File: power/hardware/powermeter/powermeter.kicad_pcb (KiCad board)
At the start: 2 copper layers, 34.6 x 35.6 mm, 20 parts, among them J1 Conn_01x02_Socket, J2 Conn_01x04_Pin, J3 Conn_01x02_Socket, P1 USB_C_Plug_USB2.0, U2 ESP32-S3-WROOM-1, U3 AZ1117-3.3

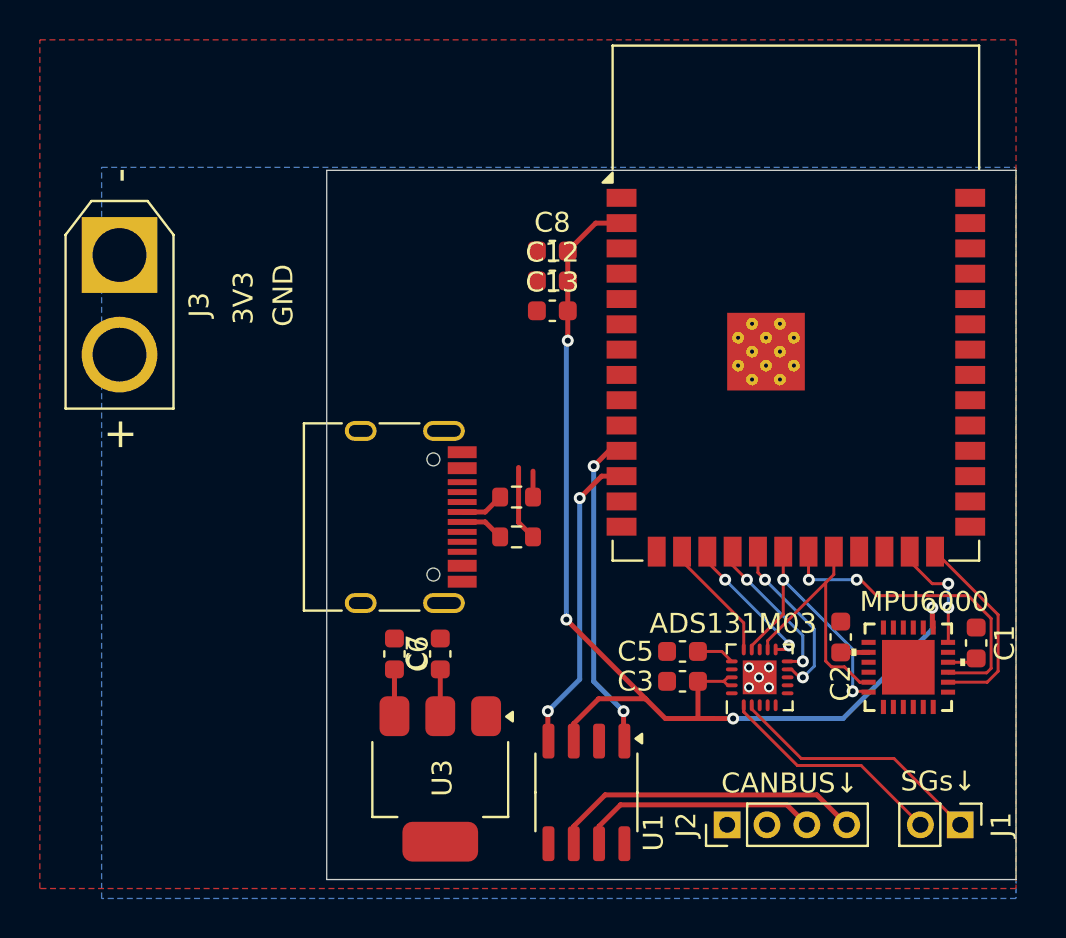
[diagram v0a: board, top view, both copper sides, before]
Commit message: updated pcb
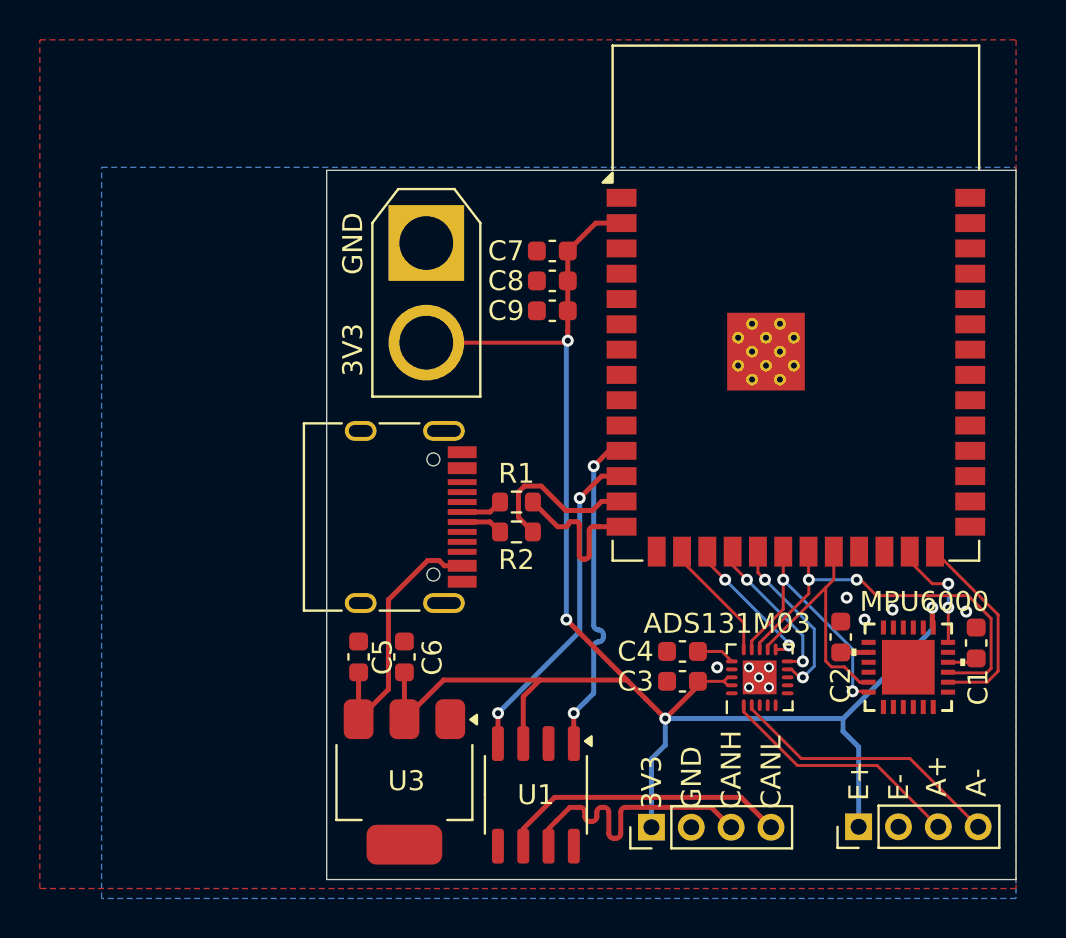
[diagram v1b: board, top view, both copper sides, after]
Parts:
- removed J1: Conn_01x02_Socket, Connector_PinHeader_2.00mm:PinHeader_1x02_P2.00mm_Vertical
- added J4: Conn_01x04_Pin, Connector_PinHeader_2.00mm:PinHeader_1x04_P2.00mm_Vertical, F.Cu at (181.5, 89.9)
- moved J3 15.4 mm to (159.8, 60.6)
- moved J2 3.80 mm to (171.1, 89.9)
- moved U1 2.54 mm to (165.3, 88.3)
- moved C6 1.81 mm to (158.7, 81.4)
- moved U3 1.81 mm to (158.7, 87.7)
- moved C5 1.81 mm to (156.4, 81.4)
- moved R1 0.25 mm to (164.3, 73.6)
- moved R2 0.25 mm to (164.3, 75.1)
- renumbered C5 to C4, C6 to C5, C7 to C6, C8 to C7, C12 to C8, C13 to C9
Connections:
- ADS131M03 pad 21: (no net) -> GND
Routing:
- net +3V3: track 58.1 -> 87.1 mm
- net +5V: track 2.49 -> 13.6 mm
- net /USB_{D}+: track 1.30 -> 8.26 mm
- net /MISO: track 16.1 -> 20.7 mm
- net /USB_{D}-: track 3.79 -> 8.30 mm
- net /CANL: track 15.8 -> 13.7 mm
- net /RX: track 14.8 -> 16.6 mm
- net /CANH: track 12.2 -> 13.6 mm
- net /TX: track 15.6 -> 16.6 mm
- net /ADS+: track 11.5 -> 12.5 mm
- net /ADS-: track 13.1 -> 14.0 mm
- net GND: track 0.00 -> 0.04 mm, vias 5 -> 10
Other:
- board text added: "3 power sources: - 5V USB - 3.3V wired - external battery"
- board text added: "A+"
- board text added: "A-"
- board text added: "CANH"
- board text added: "CANL"
- board text added: "E+"
- board text added: "E-"
- board text added: "is AdS131 vdd And dvdd TgT ok? is connecting all the power sources and using the same decoupling capacitors ok?? regardless, make sure u have all the decoupling capacitors u need --> how do we know which capacitor to use? which frequency to get rid of? make edges rounded + add mounting points? make more compact..? add silkscreen add 3d models need voltage + ground out wires for wsb?? add protecti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"
- board text removed: "CANBUS↓"
- board text removed: "SGs↓"
- board text removed: "is AdS131 vdd And dvdd TgT ok? is connecting all the power sources and using the same decoupling capacitors ok?? regardless, make sure u have all the decoupling capacitors u need --> how do we know which capacitor to use? which frequency to get rid of? make edges rounded + add mounting points? make more compact..? add silkscreen, JLCJLCJLCJLC add 3d models need voltage + ground out wires for wsb?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"
